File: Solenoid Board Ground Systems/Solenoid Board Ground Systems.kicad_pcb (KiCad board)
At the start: 2 copper layers, 63.5 x 25.4 mm, 32 parts, among them J1 OUT CHAN 1, J2 IN CHAN 1, J3 OUT CHAN 2, J4 IN CHAN 2

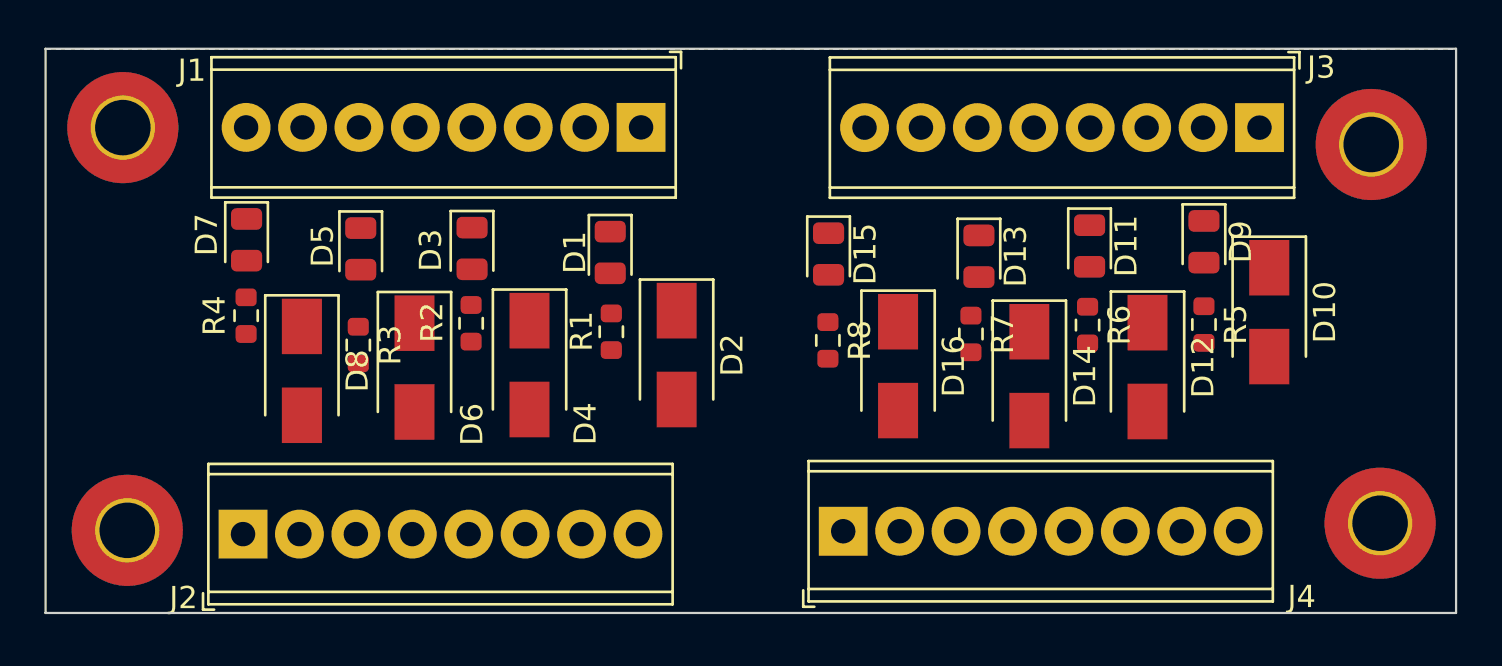
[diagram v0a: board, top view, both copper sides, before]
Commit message: Open
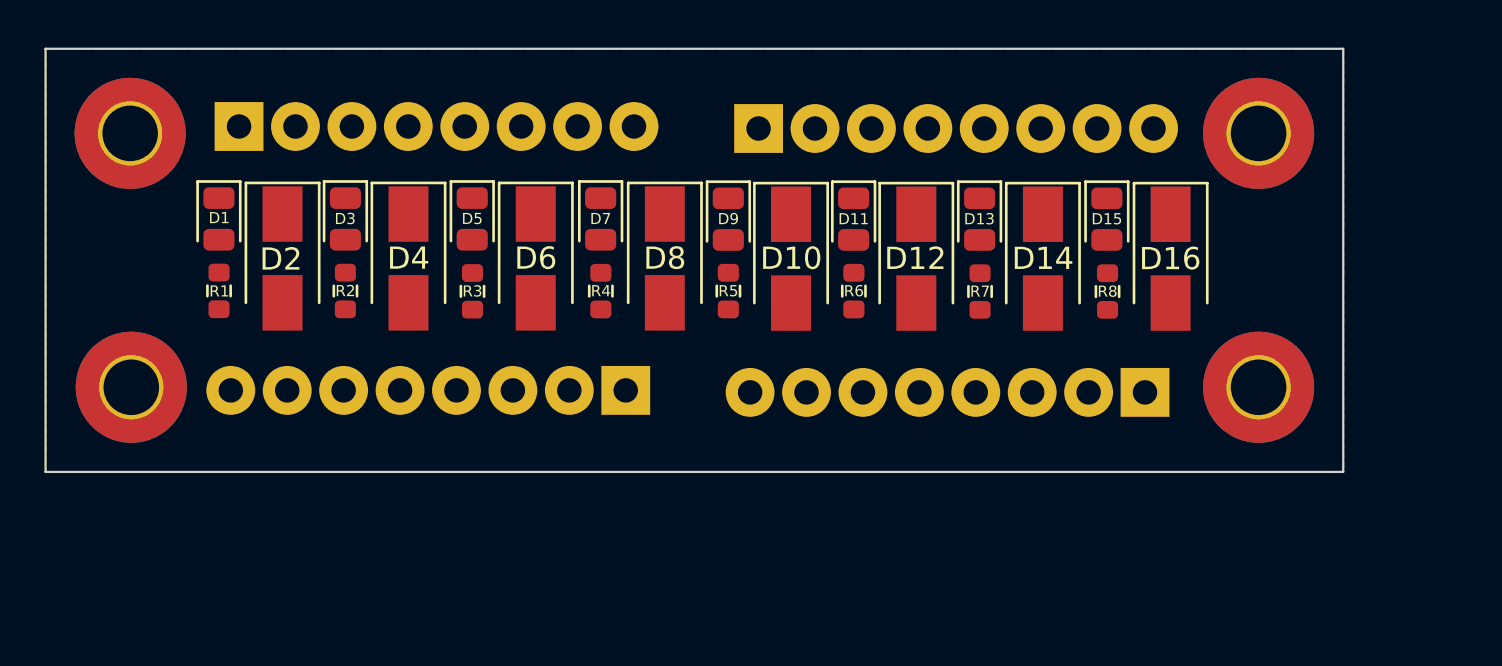
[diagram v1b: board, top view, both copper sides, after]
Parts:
- J1, J2, J3, J4: moved to B.Cu
- moved J3 22.6 mm to (57.5, 29.0), turned to 0 degrees
- moved D10 21.7 mm to (59.0, 34.9)
- moved R5 21.5 mm to (56.1, 36.3)
- moved D9 21.4 mm to (56.1, 33.1)
- moved J2 18.4 mm to (51.5, 40.8), turned to 180 degrees
- moved D2 18.3 mm to (36.1, 34.8)
- moved J1 18.1 mm to (34.1, 28.9), turned to 0 degrees
- moved R1 17.8 mm to (33.2, 36.3)
- moved D1 17.7 mm to (33.2, 33.1)
- moved D8 17.1 mm to (53.3, 34.8)
- moved R4 16.0 mm to (50.4, 36.3)
- moved D7 16.0 mm to (50.4, 33.1)
- moved J4 15.0 mm to (74.9, 40.9), turned to 180 degrees
- moved D16 13.2 mm to (76.0, 34.9)
- moved R8 12.8 mm to (73.2, 36.3)
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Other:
- board size 63.5 x 25.4 mm -> 58.4 x 19.1 mm
